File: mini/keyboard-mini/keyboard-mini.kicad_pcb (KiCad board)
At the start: 2 copper layers, 100 x 70 mm, 37 parts, among them J2 IO

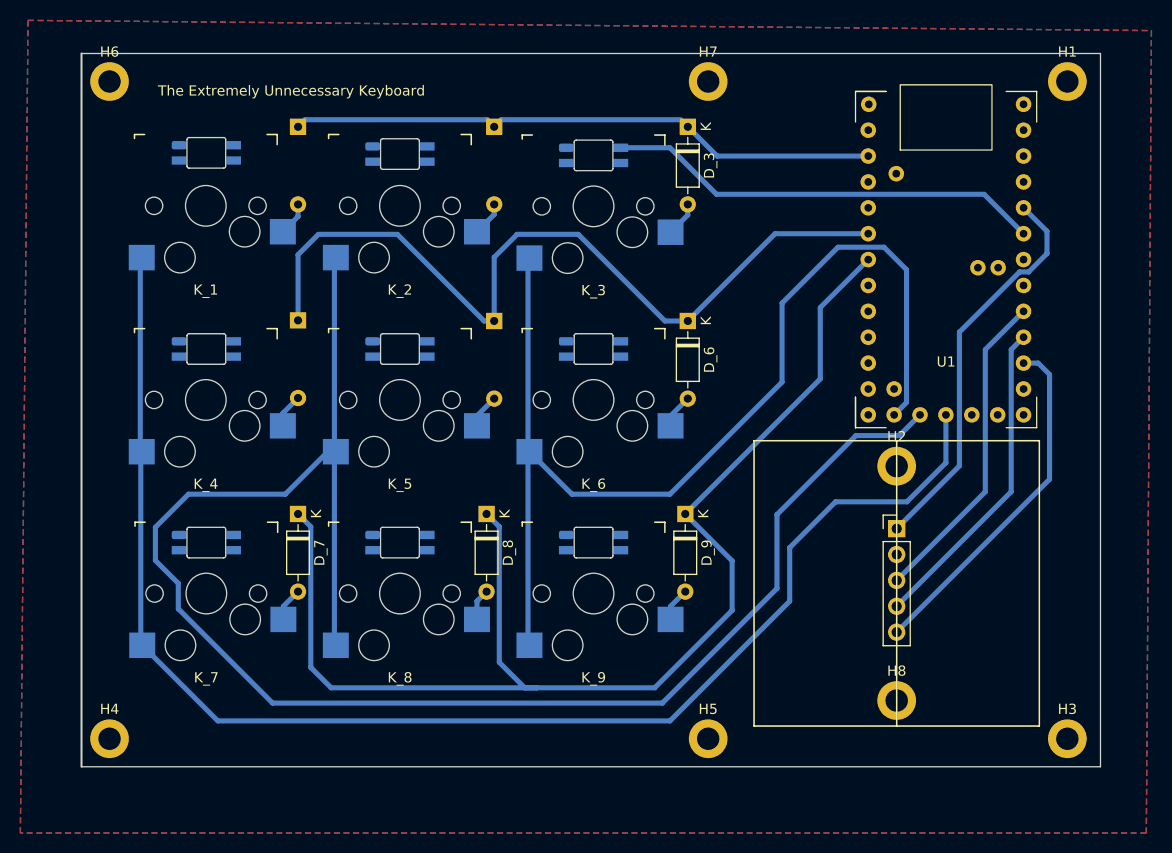
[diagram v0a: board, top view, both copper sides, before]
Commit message: mini
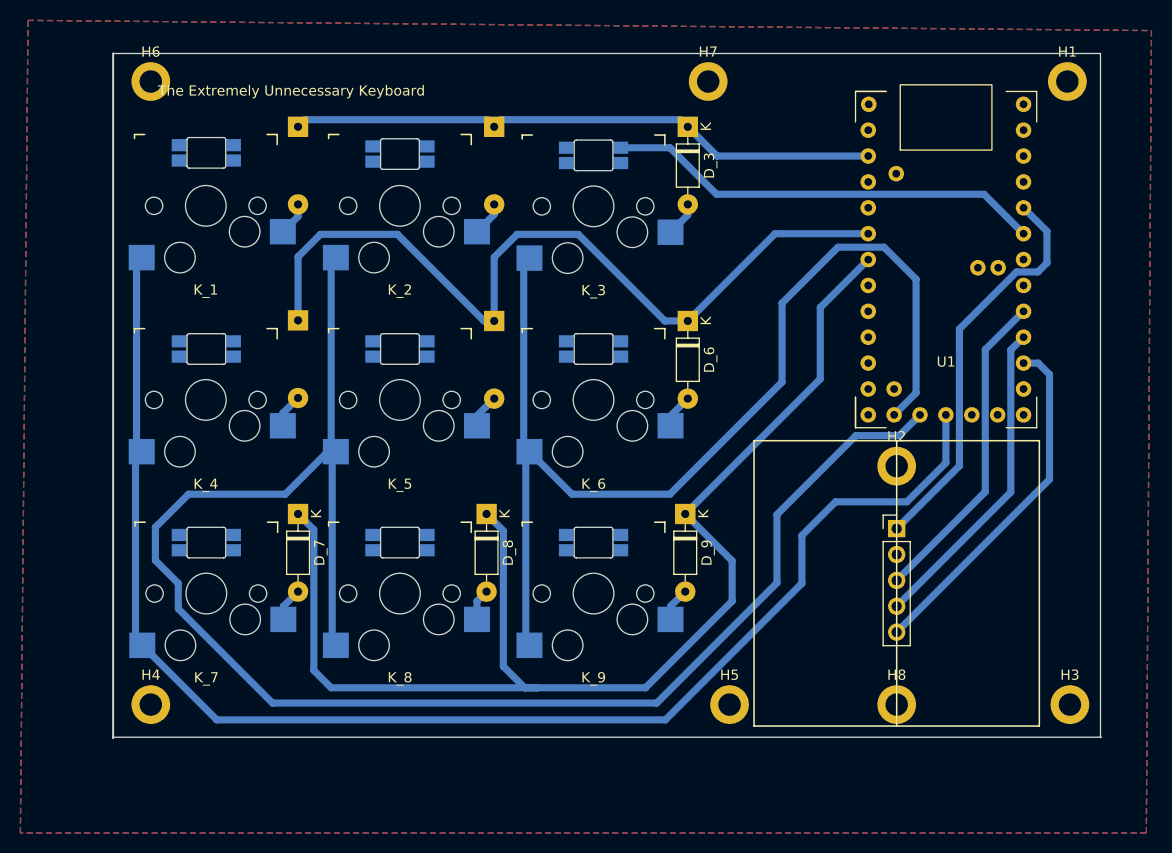
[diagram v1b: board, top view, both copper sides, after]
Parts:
- D_1, D_2, D_3, D_4, D_5, D_6, D_7, D_8, D_9: footprint Diode_THT:D_DO-35_SOD27_P7.62mm_Horizontal -> EUK:D_DO-35_SOD27_P7.62mm_Horizontal
- moved H4 5.26 mm to (184.8, 193.9)
- moved H6 4.05 mm to (184.8, 132.8)
- moved H5 3.95 mm to (241.6, 193.9)
- moved H3 3.36 mm to (275.0, 193.9)
- moved H8 0.40 mm to (258.0, 193.9)
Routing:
- net col2: track 107.2 -> 108.5 mm
- net 3V3: track 39.1 -> 39.8 mm
- net row2: track 124.5 -> 124.0 mm
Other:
- board size 100 x 70 mm -> 97 x 67.2 mm

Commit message: fixes
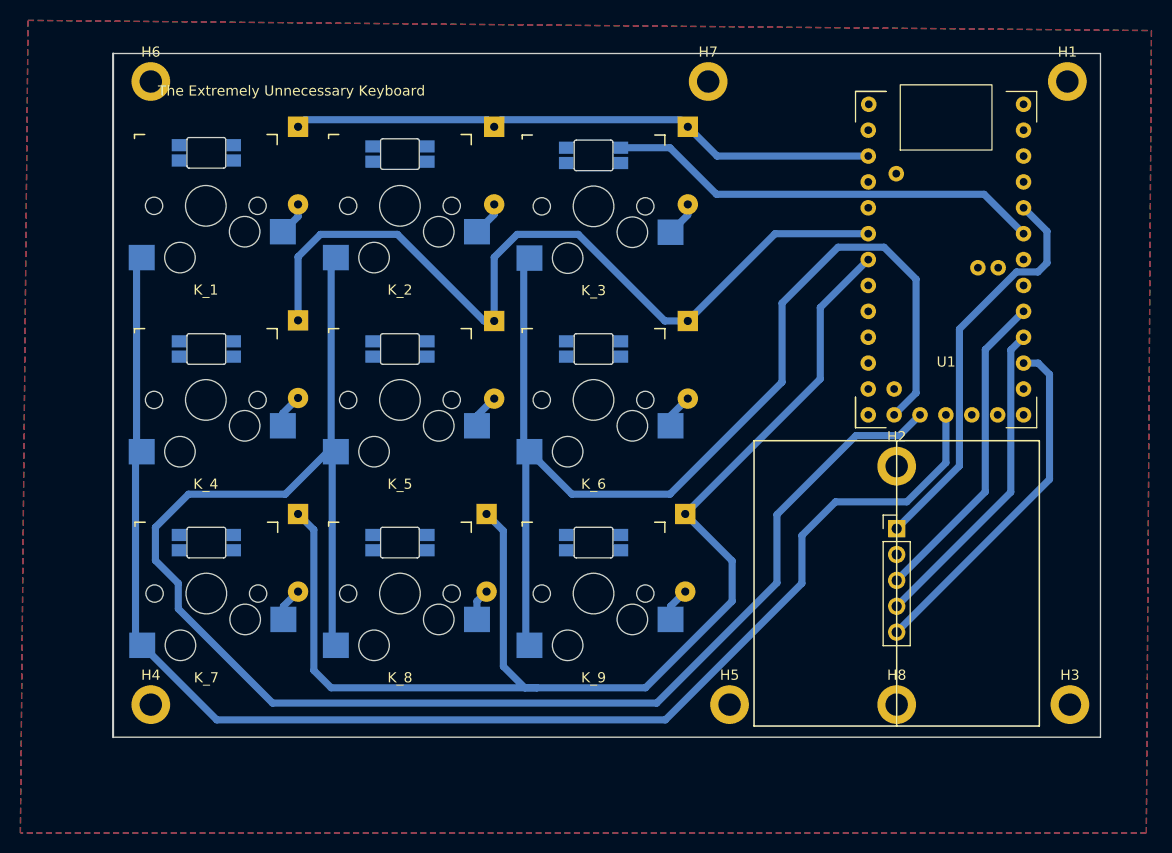
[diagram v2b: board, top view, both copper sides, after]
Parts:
- D_3, D_6, D_7, D_8, D_9: moved to B.Cu
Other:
- board size 97 x 67.2 mm -> 96.9 x 67.1 mm
